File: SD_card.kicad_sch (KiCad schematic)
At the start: 3 parts, among them J3 Micro_SD_Card_Det_Hirose_DM3AT

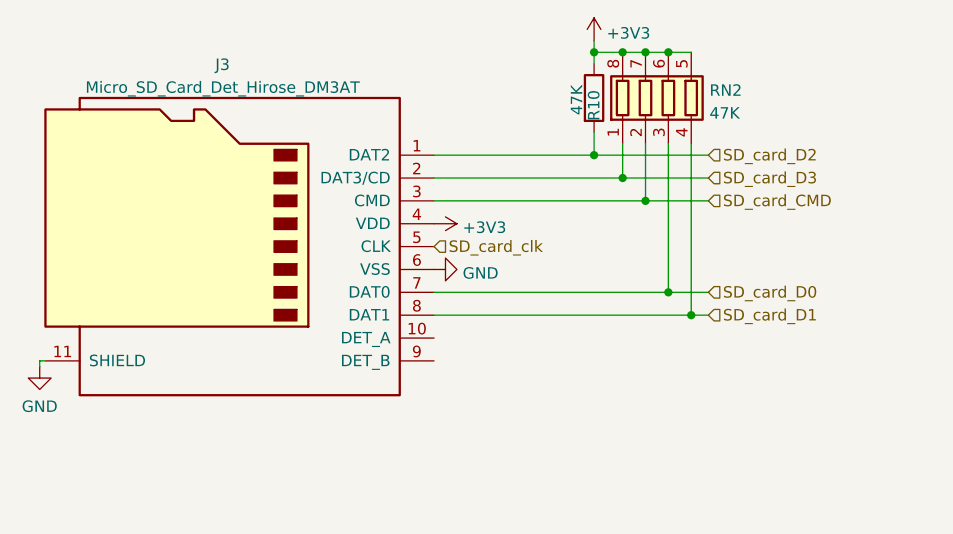
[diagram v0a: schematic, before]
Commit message: almost done
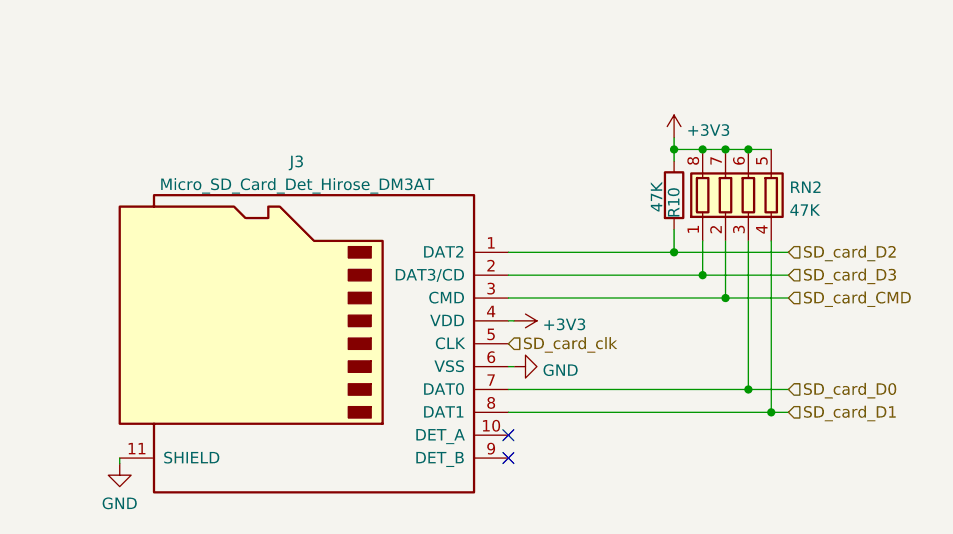
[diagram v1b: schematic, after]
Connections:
- no-connect marks 0 -> 2
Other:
- moved on the sheet: J3, R10, RN2
